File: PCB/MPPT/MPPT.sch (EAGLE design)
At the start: 25 parts, among them IC3 ACS711KEXLT-15AB-T, IC4 ACS711KEXLT-15AB-T

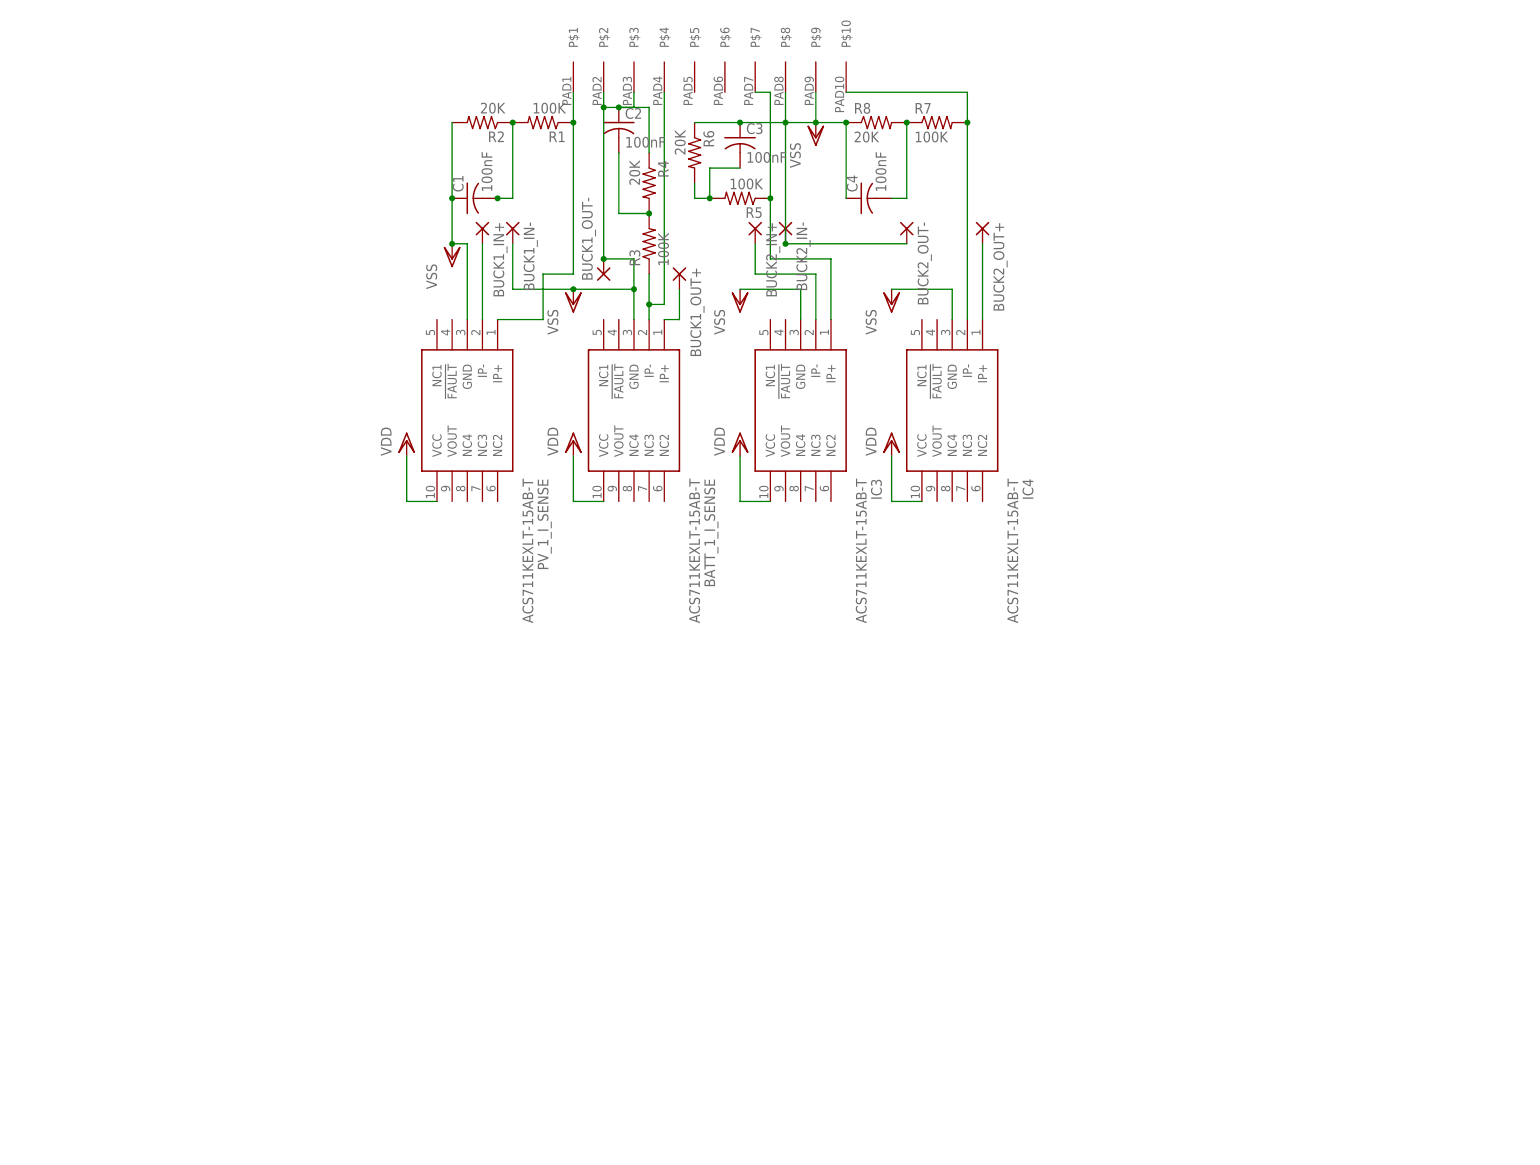
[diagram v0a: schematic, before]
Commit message: BP
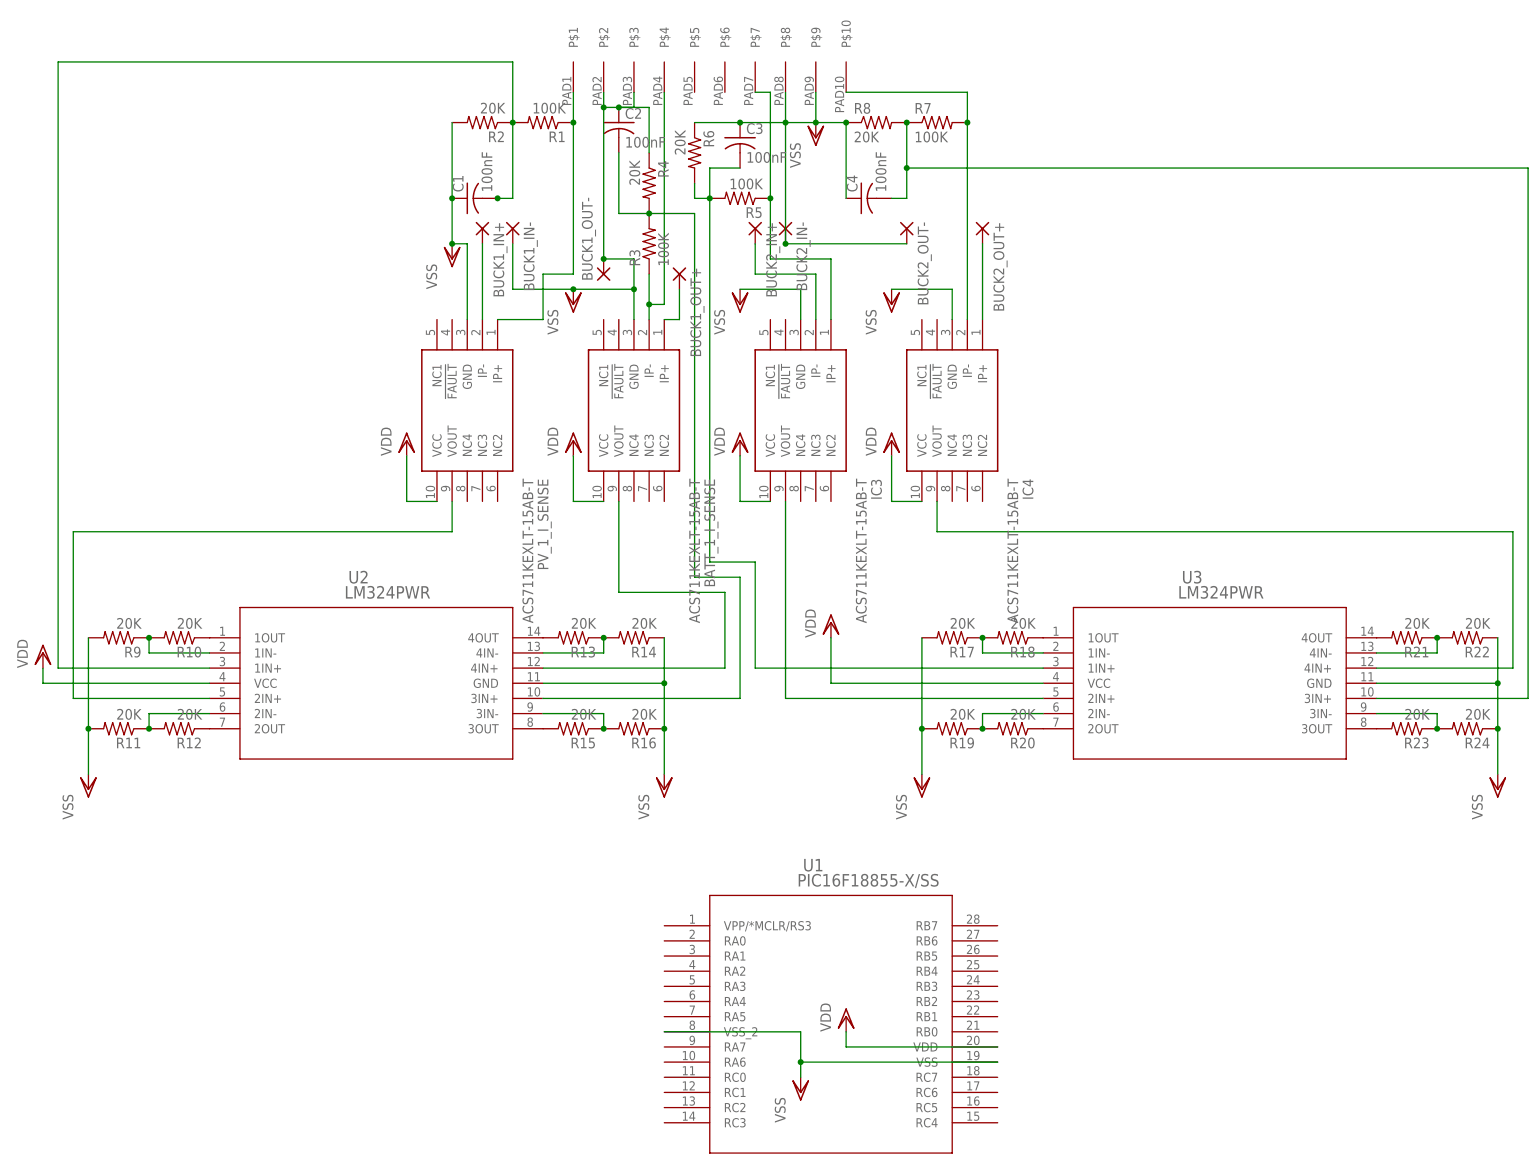
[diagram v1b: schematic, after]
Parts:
- added R10, R11, R12, R13, R14, R15, R16, R17, R18, R19, R20, R21, R22, R23, R24, R9: 20K, resistor:R-US_R0603
- added U1: PIC16F18855-X/SS, 16F18855_SSOP:PIC16F18855-X/SS
- added U2, U3: LM324PWR, LM324PWR:LM324PWR
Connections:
- new net N$14: R15.1, R16.2, U2.3IN-
- new net N$15: R10.1, U2.1OUT
- new net N$16: R11.1, R12.2, U2.2IN-
- new net N$17: R12.1, U2.2OUT
- new net N$18: R13.1, R14.2, U2.4IN-
- new net N$19: R10.2, R9.1, U2.1IN-
- new net N$2: PV_1_I_SENSE.VOUT, U2.2IN+
- new net N$20: R13.2, U2.4OUT
- new net N$21: R15.2, U2.3OUT
- new net N$22: BATT_1_I_SENSE.VOUT, U2.4IN+
- new net N$24: R18.1, U3.1OUT
- new net N$25: R20.1, U3.2OUT
- new net N$26: R19.1, R20.2, U3.2IN-
- new net N$27: R21.2, U3.4OUT
- new net N$28: R21.1, R22.2, U3.4IN-
- new net N$29: R23.2, U3.3OUT
- new net N$30: R23.1, R24.2, U3.3IN-
- new net N$31: R17.1, R18.2, U3.1IN-
- new net N$32: IC3.VOUT, U3.2IN+
- new net N$33: IC4.VOUT, U3.4IN+
- net N$10: now also U3.1IN+
- net N$12: now also U3.3IN+
- net N$3: now also U2.1IN+
- net N$5: now also U2.3IN+
- net VDD: now also U1.VDD, U2.VCC, U3.VCC
- net VSS: now also R11.2, R14.1, R16.1, R17.2, R19.2, R22.1, R24.1, R9.2, U1.VSS, U1.VSS_2, U2.GND, U3.GND
